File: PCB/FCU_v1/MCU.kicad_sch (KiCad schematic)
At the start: 27 parts, among them J3 Conn_01x05_Pin, SW1 SW_SPDT, U11 STM32G473RETx, Y2 16MHz

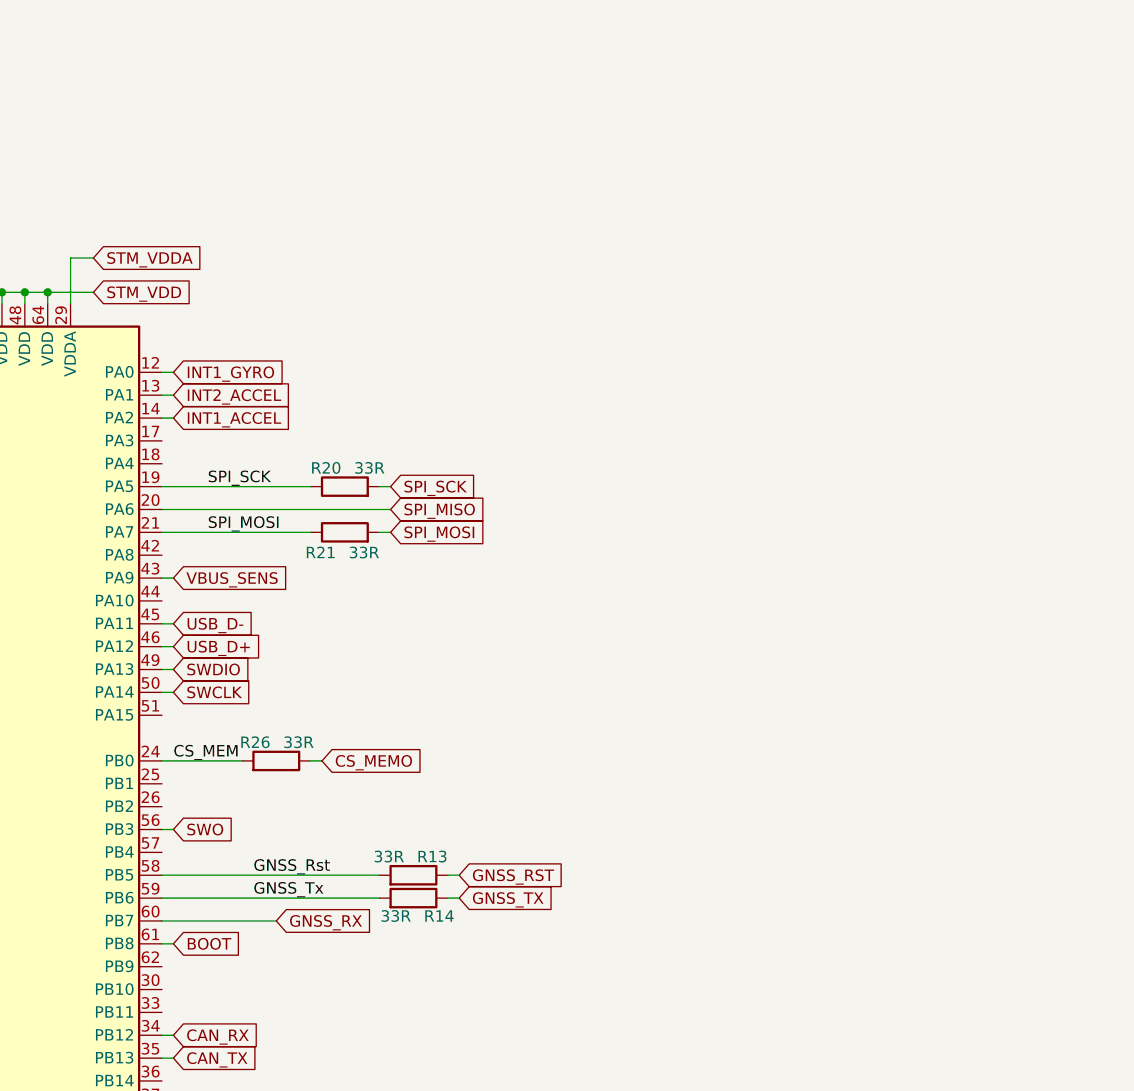
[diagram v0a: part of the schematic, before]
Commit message: Layout update
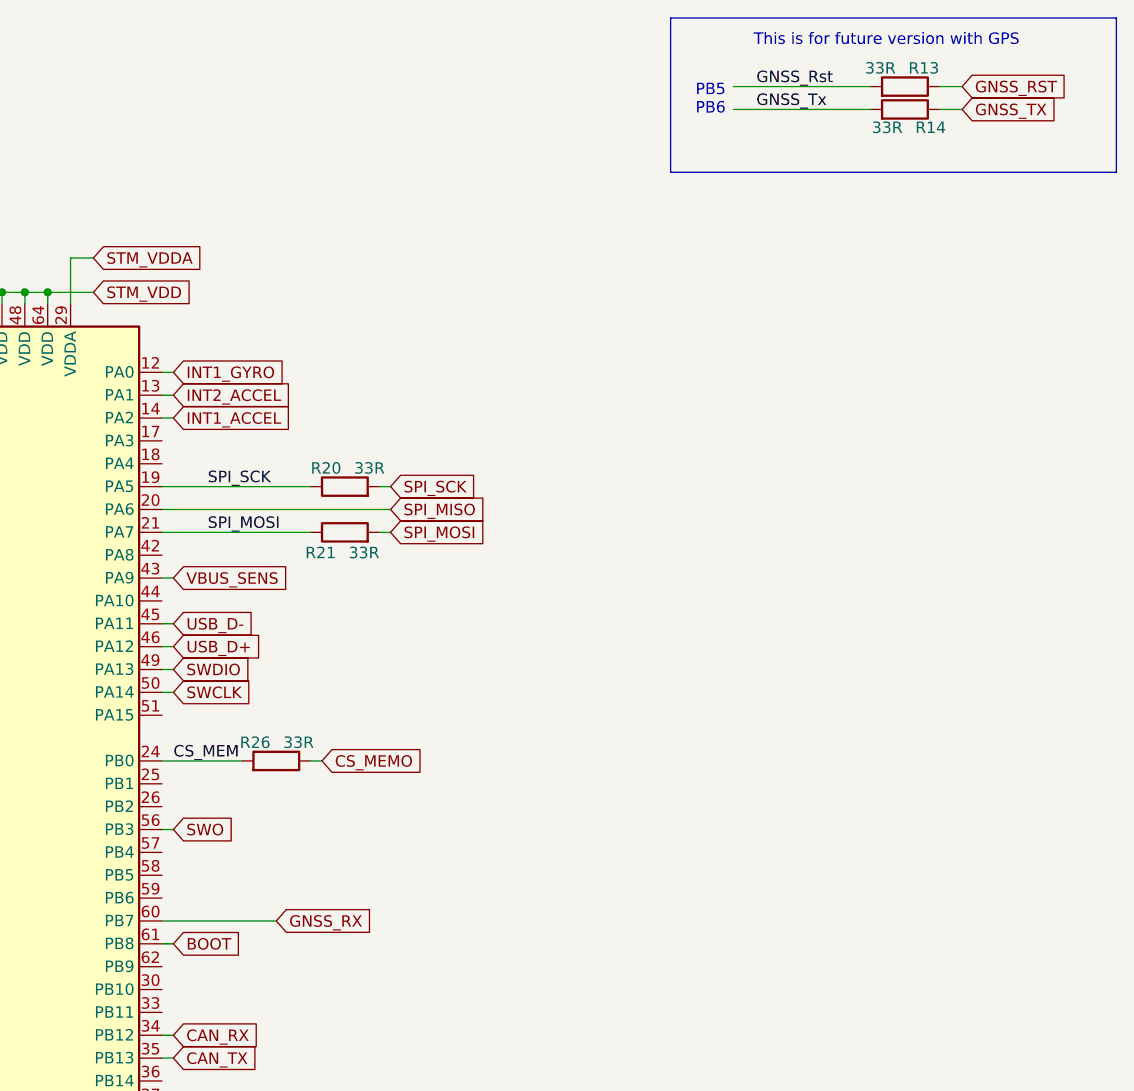
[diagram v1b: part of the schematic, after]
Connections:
- net GNSS_Rst: no longer U11.58 (PB5)
- net GNSS_Tx: no longer U11.59 (PB6)
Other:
- note added: "PB5 PB6"
- note added: "This is for future version with GPS"
- moved on the sheet: R13, R14
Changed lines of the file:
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@@
 	)
 	(rectangle
+		(start 230.505 13.97)
+		(end 280.035 31.115)
+		(stroke
+			(width 0)
+			(type default)
+		)
+		(fill
+			(type none)
+		)
+	)
+	(rectangle
 		(start 16.51 59.69)
 		(end 52.07 85.09)
@@
 		)
 	)
+	(text "This is for future version with GPS"
+		(exclude_from_sim no)
+		(at 254.508 16.51 0)
+		(effects
+			(font
+				(size 1.27 1.27)
+			)
+		)
+	)
+	(text "PB5\nPB6"
+		(exclude_from_sim no)
+		(at 234.95 23.114 0)
+		(effects
+			(font
+				(size 1.27 1.27)
+			)
+		)
+	)
 	(text "SWD"
 		(exclude_from_sim no)
@@
 	(wire
 		(pts
+			(xy 237.49 21.59) (xy 252.73 21.59)
+		)
+		(stroke
+			(width 0)
+			(type default)
+		)
+	)
+	(wire
+		(pts
 			(xy 45.72 34.29) (xy 45.72 33.02)
 		)
@@
 	(wire
 		(pts
-			(xy 207.01 109.22) (xy 205.74 109.22)
+			(xy 262.89 21.59) (xy 260.35 21.59)
 		)
 		(stroke
@@
 	(wire
 		(pts
-			(xy 173.99 109.22) (xy 198.12 109.22)
-		)
-		(stroke
-			(width 0)
-			(type default)
-		)
-	)
-	(wire
-		(pts
 			(xy 151.13 44.45) (xy 151.13 45.72)
 		)
@@
 	(wire
 		(pts
-			(xy 207.01 111.76) (xy 205.74 111.76)
+			(xy 262.89 24.13) (xy 260.35 24.13)
 		)
 		(stroke
@@
 	(wire
 		(pts
+			(xy 237.49 24.13) (xy 252.73 24.13)
+		)
+		(stroke
+			(width 0)
+			(type default)
+		)
+	)
+	(wire
+		(pts
 			(xy 116.84 96.52) (xy 124.46 96.52)
 		)
@@
 	(wire
 		(pts
-			(xy 173.99 111.76) (xy 198.12 111.76)
-		)
-		(stroke
-			(width 0)
-			(type default)
-		)
-	)
-	(wire
-		(pts
 			(xy 39.37 53.34) (xy 39.37 54.61)
 		)
@@
 	)
 	(label "GNSS_Tx"
-		(at 184.15 111.76 0)
+		(at 240.03 24.13 0)
 		(effects
 			(font
@@
 	)
 	(label "GNSS_Rst"
-		(at 184.15 109.22 0)
+		(at 240.03 21.59 0)
 		(effects
 			(font
@@
 	(global_label "GNSS_RST"
 		(shape input)
-		(at 207.01 109.22 0)
+		(at 262.89 21.59 0)
 		(fields_autoplaced yes)
 		(effects
@@
 		)
 		(property "Intersheetrefs" "${INTERSHEET_REFS}"
-			(at 219.4294 109.22 0)
+			(at 275.3094 21.59 0)
 			(effects
 				(font
@@
 	(global_label "GNSS_TX"
 		(shape input)
-		(at 207.01 111.76 0)
+		(at 262.89 24.13 0)
 		(fields_autoplaced yes)
 		(effects
@@
 		)
 		(property "Intersheetrefs" "${INTERSHEET_REFS}"
-			(at 218.1594 111.76 0)
+			(at 274.0394 24.13 0)
 			(effects
 				(font
@@
 	(symbol
 		(lib_id "Device:R")
-		(at 201.93 111.76 270)
+		(at 256.54 24.13 270)
 		(mirror x)
 		(unit 1)
@@
 		(dnp no)
 		(property "Reference" "R14"
-			(at 206.502 113.792 90)
+			(at 261.112 26.162 90)
 			(effects
 				(font
@@
 		)
 		(property "Value" "33R"
-			(at 201.676 113.792 90)
+			(at 256.286 26.162 90)
 			(effects
 				(font
@@
 		)
 		(property "Footprint" "Resistor_SMD:R_0603_1608Metric"
-			(at 201.93 113.538 90)
+			(at 256.54 25.908 90)
 			(effects
 				(font
@@
 		)
 		(property "Datasheet" "~"
-			(at 201.93 111.76 0)
+			(at 256.54 24.13 0)
 			(effects
 				(font
@@
 		)
 		(property "Description" "Resistor"
-			(at 201.93 111.76 0)
+			(at 256.54 24.13 0)
 			(effects
 				(font
@@
 	(symbol
 		(lib_id "Device:R")
-		(at 201.93 109.22 270)
+		(at 256.54 21.59 270)
 		(mirror x)
 		(unit 1)
@@
 		(dnp no)
 		(property "Reference" "R13"
-			(at 205.74 107.188 90)
+			(at 260.35 19.558 90)
 			(effects
 				(font
@@
 		)
 		(property "Value" "33R"
-			(at 200.914 107.188 90)
+			(at 255.524 19.558 90)
 			(effects
 				(font
@@
 		)
 		(property "Footprint" "Resistor_SMD:R_0603_1608Metric"
-			(at 201.93 110.998 90)
+			(at 256.54 23.368 90)
 			(effects
 				(font
@@
 		)
 		(property "Datasheet" "~"
-			(at 201.93 109.22 0)
+			(at 256.54 21.59 0)
 			(effects
 				(font
@@
 		)
 		(property "Description" "Resistor"
-			(at 201.93 109.22 0)
+			(at 256.54 21.59 0)
 			(effects
 				(font

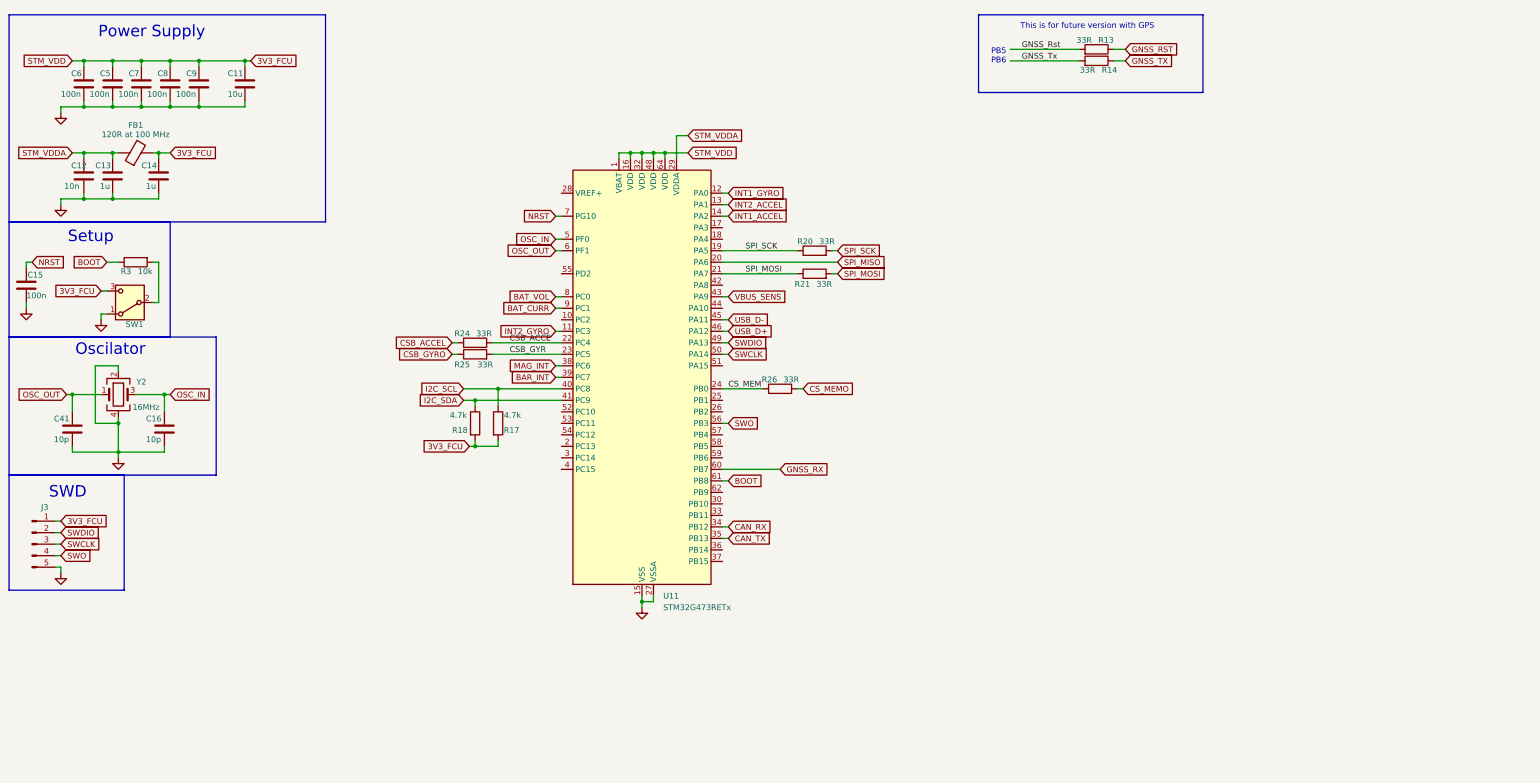
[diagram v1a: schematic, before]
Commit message: Schematic update
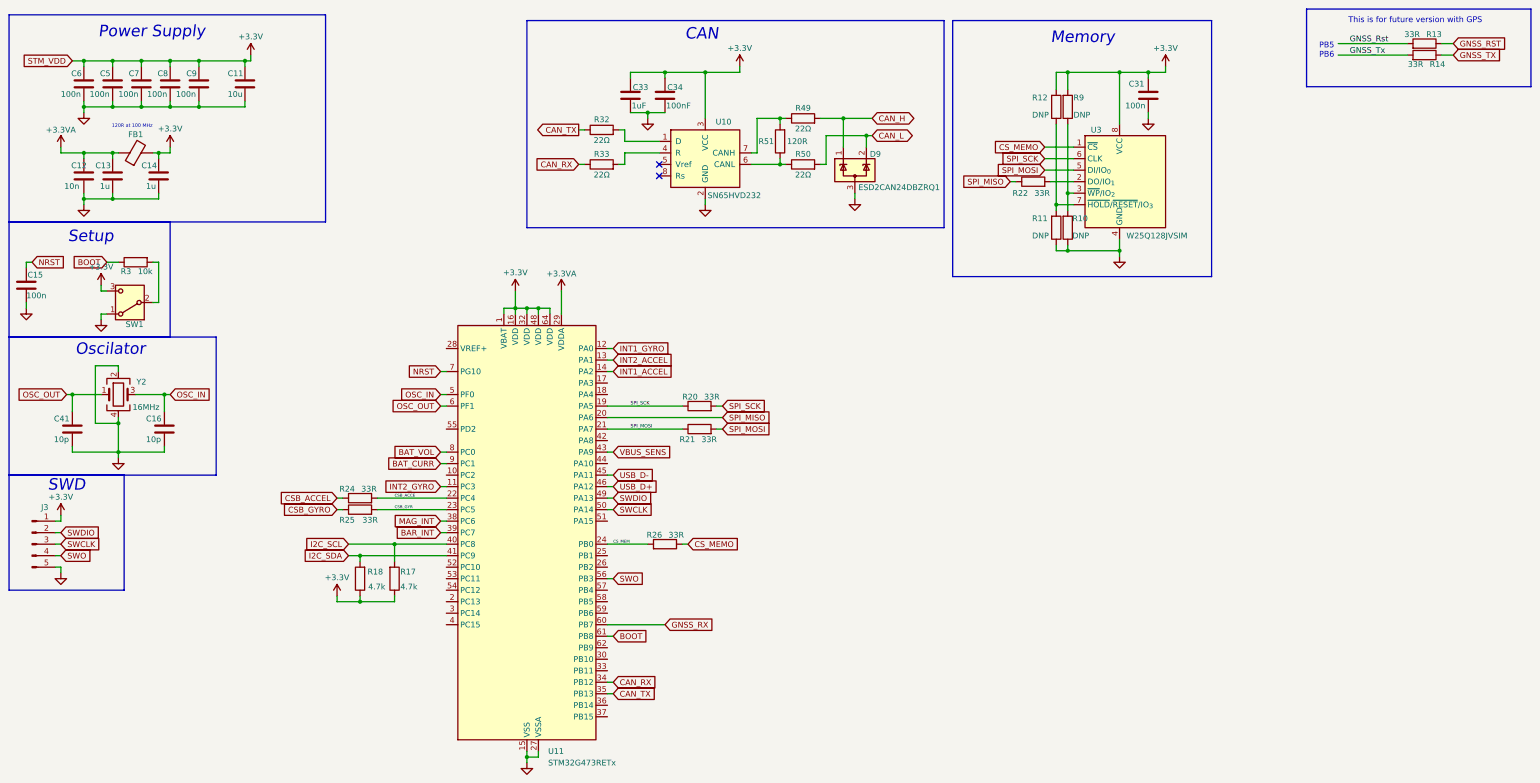
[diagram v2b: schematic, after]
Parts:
- added C31: 100n, Capacitor_SMD:C_0805_2012Metric, symbol Device:C
- added C33: 1uF, Capacitor_SMD:C_0805_2012Metric, symbol Device:C
- added C34: 100nF, Capacitor_SMD:C_0805_2012Metric, symbol Device:C
- added D9: ESD2CAN24DBZRQ1, Package_TO_SOT_SMD:SOT-23-3, symbol Power_Protection:ESDA5V3L
- added R10, R11, R12, R9: DNP, Resistor_SMD:R_0201_0603Metric, symbol Device:R
- added R22: 33R, Resistor_SMD:R_0603_1608Metric, symbol Device:R
- added R32, R33, R49, R50: 22Ω, Resistor_SMD:R_0603_1608Metric, symbol Device:R
- added R51: 120R, Resistor_SMD:R_0603_1608Metric, symbol Device:R
- added U10: SN65HVD232, Package_SO:SOIC-8_3.9x4.9mm_P1.27mm, symbol Interface_CAN_LIN:SN65HVD230
- added U3: W25Q128JVSIM, Package_SO:SOIC-8_5.3x5.3mm_P1.27mm, symbol Memory_Flash:W25Q128JVS
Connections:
- net CAN_RX: now also R33.1
- net CAN_TX: now also R32.1
- net CS_MEMO: now also U3.1 (~{CS})
- net GND: now also C31.2, C33.2, C34.2, D9.3 (A), R10.1, R11.1, U10.2 (GND), U3.4 (GND)
- net I2C_SCL: now also R17.2; no longer R17.1
- net I2C_SDA: now also R18.2; no longer R18.1
- net SPI_MISO: now also R22.1
- net SPI_MOSI: now also U3.5 (DI/IO_{0})
- net SPI_SCK: now also U3.6 (CLK)
- net 3V3_FCU renamed +3.3V
- net +3.3V: now also R17.1, R18.1, C31.1, C33.1, C34.1, R12.2, R9.2, U10.3 (VCC), U3.8 (VCC); no longer R17.2, R18.2
- net STM_VDDA renamed +3.3VA
- new net: R50.1, R51.1, U10.6 (CANL)
- new net: R49.1, R51.2, U10.7 (CANH)
- new net: R11.2, R12.1, U3.7 (~{HOLD}/~{RESET}/IO_{3})
- new net: R10.2, R9.1, U3.3 (~{WP}/IO_{2})
- new net: R33.2, U10.4 (R)
- new net: R32.2, U10.1 (D)
- new net: R22.2, U3.2 (DO/IO_{1})
- new net CAN_H: D9.1 (K), R49.2
- new net CAN_L: D9.2 (K), R50.2
- no-connect marks 0 -> 2
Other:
- note added: "120R at 100 MHz"
- note added: "CAN"
- note added: "Memory"
- moved on the sheet: R13, R14, R17, R18, R20, R21, R24, R25, R26, U11
